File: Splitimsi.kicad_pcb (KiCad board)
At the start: 2 copper layers, 118.2 x 99.3 mm, 30 parts, among them SW1 MX_RGB, SW10 MX_RGB, SW11 MX_RGB, SW12 MX_RGB, SW13 MX_RGB, SW14 MX_RGB, SW15 MX_RGB, SW16 MX_RGB, SW17 MX_RGB, SW18 MX_RGB, SW19 MX_RGB, SW2 MX_RGB, SW20 MX_RGB, SW21 MX_RGB, SW22 MX_RGB, SW23 MX_RGB, SW24 MX_RGB, SW25 MX_RGB, SW26 MX_RGB, SW27 MX_RGB, SW3 MX_RGB, SW4 MX_RGB, SW5 MX_RGB, SW6 MX_RGB, SW7 MX_RGB, SW8 MX_RGB, SW9 MX_RGB, U1 ProMicro, U2 TRRS

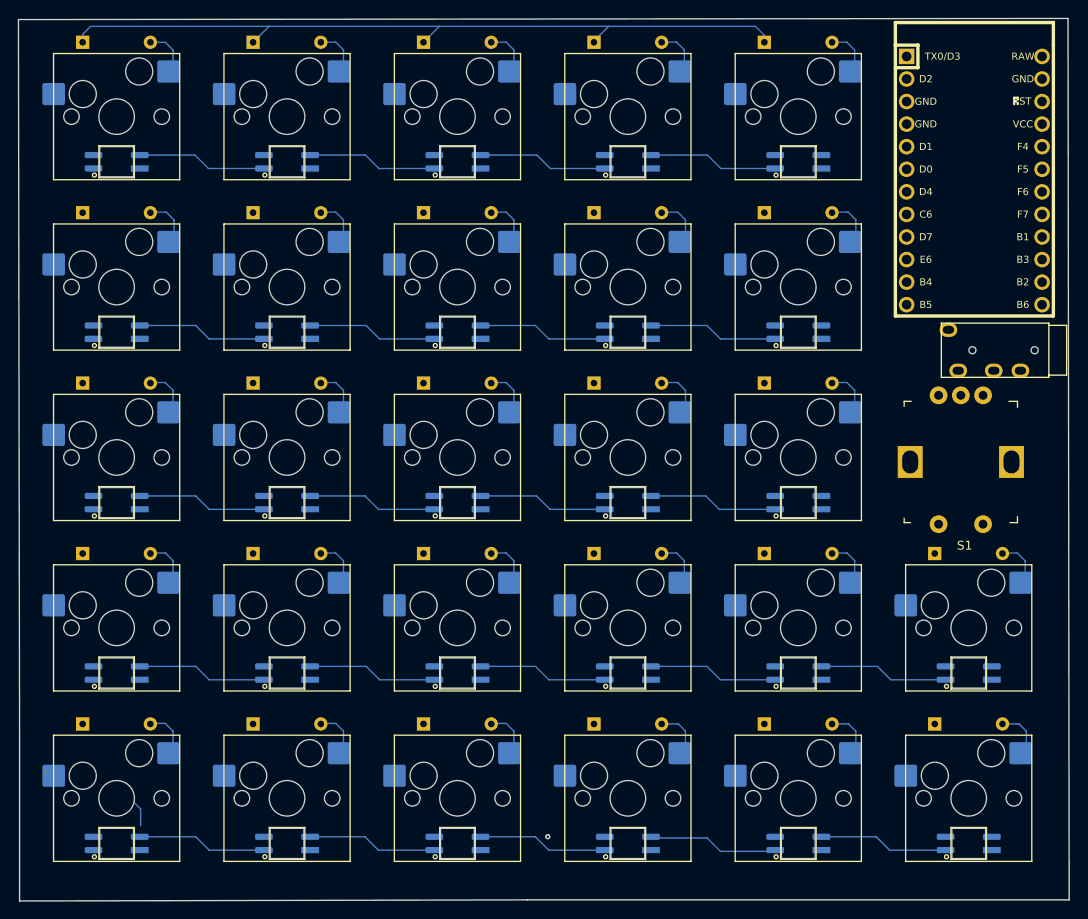
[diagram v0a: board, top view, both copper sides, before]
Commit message: Minor Adjustments
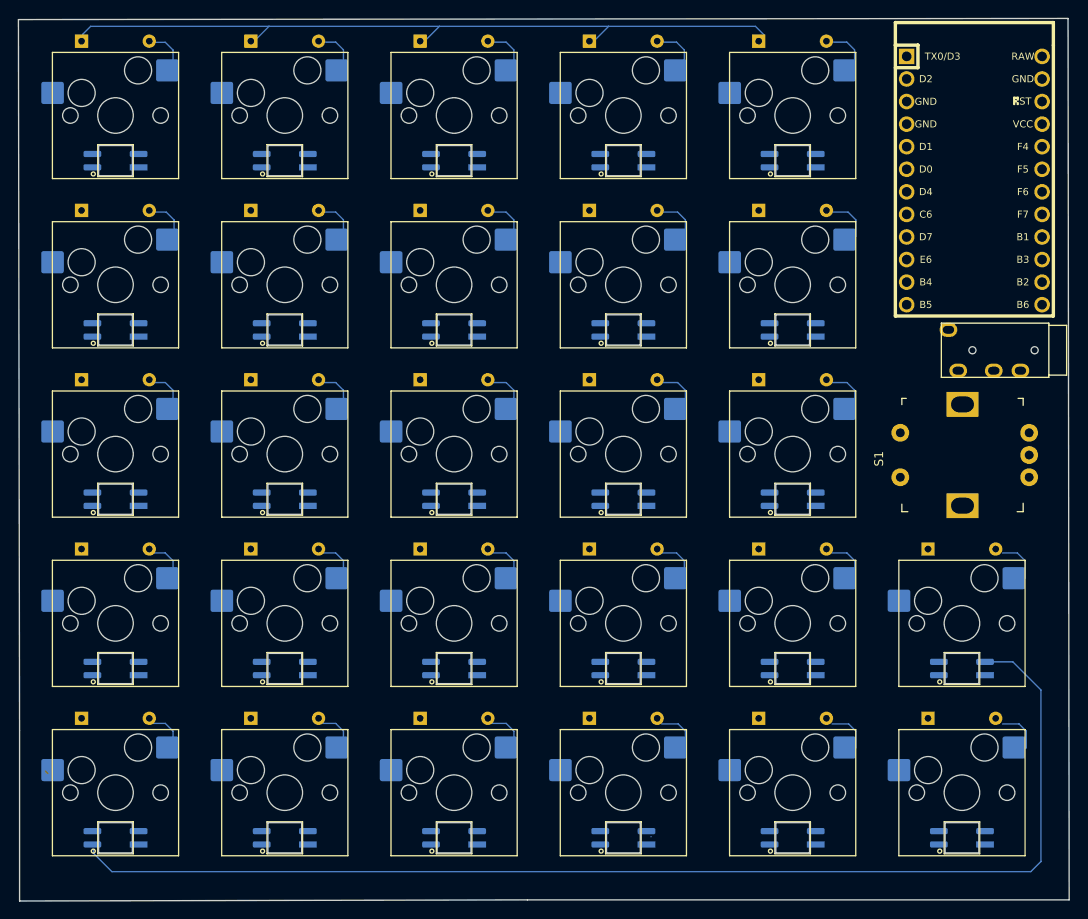
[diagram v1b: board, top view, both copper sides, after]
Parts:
- moved S1 7.39 mm to (126.4, 72.5), turned to 90 degrees
- moved SW27 0.99 mm to (127.0, 104.8)
- moved SW21 0.92 mm to (127.0, 85.7)
- moved SW26 0.90 mm to (108.0, 104.8)
- moved SW20 0.81 mm to (108.0, 85.7)
- moved SW25 0.81 mm to (88.9, 104.8)
- moved SW15 0.74 mm to (108.0, 66.7)
- moved SW24 0.74 mm to (69.8, 104.8)
- moved SW19 0.72 mm to (88.9, 85.7)
- moved SW23 0.68 mm to (50.8, 104.8)
- moved SW10 0.68 mm to (108.0, 47.6)
- moved SW5 0.65 mm to (108.0, 28.6)
- moved SW22 0.65 mm to (31.8, 104.8)
- moved SW18 0.64 mm to (69.8, 85.7)
- moved SW14 0.63 mm to (88.9, 66.7)
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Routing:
- net Net-(SW21-Pad6): track 0.00 -> 135.2 mm
- net Net-(SW24-Pad6): track 14.8 -> 0.00 mm, vias 1 -> 0
- net Net-(SW4-Pad6): track 14.6 -> 0.00 mm
- net Net-(SW3-Pad6): track 14.6 -> 0.00 mm
- net Net-(SW26-Pad6): track 14.6 -> 0.00 mm
- net Net-(SW23-Pad6): track 14.6 -> 0.00 mm
- net Net-(SW22-Pad6): track 14.6 -> 0.00 mm
- net Net-(SW20-Pad6): track 14.6 -> 0.00 mm
- net Net-(SW2-Pad6): track 14.6 -> 0.00 mm
- net Net-(SW18-Pad6): track 14.6 -> 0.00 mm
- net Net-(SW16-Pad6): track 14.6 -> 0.00 mm
- net Net-(SW14-Pad6): track 14.6 -> 0.00 mm
- net Net-(SW13-Pad6): track 14.6 -> 0.00 mm
- net Net-(SW11-Pad6): track 14.6 -> 0.00 mm
- net Net-(SW1-Pad6): track 14.6 -> 0.00 mm
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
